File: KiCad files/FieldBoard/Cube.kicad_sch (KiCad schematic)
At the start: 9 parts

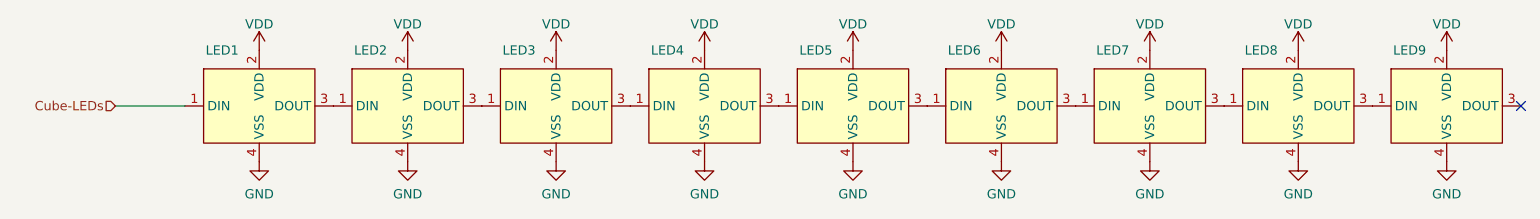
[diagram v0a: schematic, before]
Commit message: update
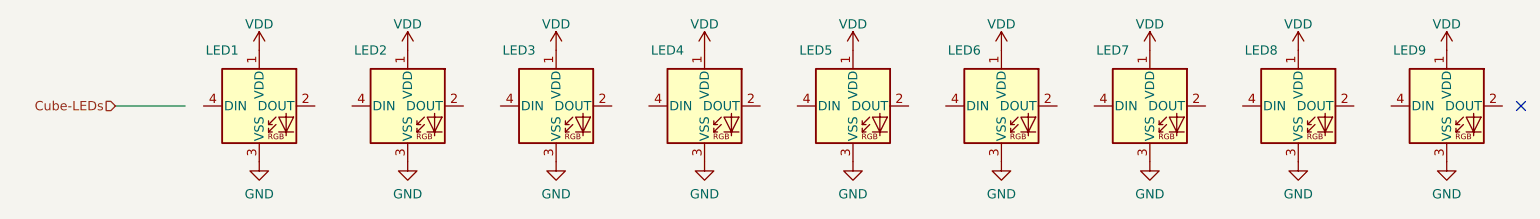
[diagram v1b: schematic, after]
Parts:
- LED1: value WS2812-4020_single -> (none); footprint FieldBoard_footprint:WS2812-4020-single-6mm_bezMaske -> LED_SMD:LED_WS2812B_PLCC4_5.0x5.0mm_P3.2mm; symbol FieldBoard_symbol:WS2812-4020_single -> LED:WS2812B
- LED2, LED3, LED4, LED5, LED6, LED7, LED8, LED9: footprint FieldBoard_footprint:WS2812-4020-single-6mm_bezMaske -> LED_SMD:LED_WS2812B_PLCC4_5.0x5.0mm_P3.2mm; symbol FieldBoard_symbol:WS2812-4020_single -> LED:WS2812B
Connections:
- net Cube-LEDs: no longer LED1.1 (DIN)
- net GND: now also LED1.3 (VSS), LED2.3 (VSS), LED3.3 (VSS), LED4.3 (VSS), LED5.3 (VSS), LED6.3 (VSS), LED7.3 (VSS), LED8.3 (VSS), LED9.3 (VSS); no longer LED1.4 (VSS), LED2.4 (VSS), LED3.4 (VSS), LED4.4 (VSS), LED5.4 (VSS), LED6.4 (VSS), LED7.4 (VSS), LED8.4 (VSS), LED9.4 (VSS)
- net VDD: now also LED1.1 (VDD), LED2.1 (VDD), LED3.1 (VDD), LED4.1 (VDD), LED5.1 (VDD), LED6.1 (VDD), LED7.1 (VDD), LED8.1 (VDD), LED9.1 (VDD); no longer LED1.2 (VDD), LED2.2 (VDD), LED3.2 (VDD), LED4.2 (VDD), LED5.2 (VDD), LED6.2 (VDD), LED7.2 (VDD), LED8.2 (VDD), LED9.2 (VDD)
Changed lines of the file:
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@@
     (pin "1")
   )
-  (symbol (lib_name "WS2812-4020_single_7") (lib_id "FieldBoard_symbol:WS2812-4020_single") (at 117.475 88.9 0) (unit 1)
+  (symbol (lib_id "LED:WS2812B") (at 117.475 88.9 0) (unit 1)
     (in_bom yes) (on_board yes)
     (property "Reference" "LED3" (id 0) (at 112.395 81.28 0))
@@
       (effects (font (size 1.27 1.27)) hide)
     )
-    (property "Footprint" "FieldBoard_footprint:WS2812-4020-single-6mm_bezMaske" (id 2) (at 117.475 88.9 0)
-      (effects (font (size 1.27 1.27)) hide)
-    )
-    (property "Datasheet" "" (id 3) (at 117.475 88.9 0)
-      (effects (font (size 1.27 1.27)) hide)
-    )
-    (pin "1")
-    (pin "2")
-    (pin "3")
-    (pin "4")
-  )
-  (symbol (lib_name "WS2812-4020_single_6") (lib_id "FieldBoard_symbol:WS2812-4020_single") (at 178.435 88.9 0) (unit 1)
+    (property "Footprint" "LED_SMD:LED_WS2812B_PLCC4_5.0x5.0mm_P3.2mm" (id 2) (at 118.745 96.52 0)
+      (effects (font (size 1.27 1.27)) (justify left top) hide)
+    )
+    (property "Datasheet" "https://cdn-shop.adafruit.com/datasheets/WS2812B.pdf" (id 3) (at 120.015 98.425 0)
+      (effects (font (size 1.27 1.27)) (justify left top) hide)
+    )
+    (pin "1")
+    (pin "2")
+    (pin "3")
+    (pin "4")
+  )
+  (symbol (lib_id "LED:WS2812B") (at 178.435 88.9 0) (unit 1)
     (in_bom yes) (on_board yes)
     (property "Reference" "LED6" (id 0) (at 173.355 81.28 0))
@@
       (effects (font (size 1.27 1.27)) hide)
     )
-    (property "Footprint" "FieldBoard_footprint:WS2812-4020-single-6mm_bezMaske" (id 2) (at 178.435 88.9 0)
-      (effects (font (size 1.27 1.27)) hide)
-    )
-    (property "Datasheet" "" (id 3) (at 178.435 88.9 0)
-      (effects (font (size 1.27 1.27)) hide)
-    )
-    (pin "1")
-    (pin "2")
-    (pin "3")
-    (pin "4")
-  )
-  (symbol (lib_name "WS2812-4020_single_2") (lib_id "FieldBoard_symbol:WS2812-4020_single") (at 97.155 88.9 0) (unit 1)
+    (property "Footprint" "LED_SMD:LED_WS2812B_PLCC4_5.0x5.0mm_P3.2mm" (id 2) (at 179.705 96.52 0)
+      (effects (font (size 1.27 1.27)) (justify left top) hide)
+    )
+    (property "Datasheet" "https://cdn-shop.adafruit.com/datasheets/WS2812B.pdf" (id 3) (at 180.975 98.425 0)
+      (effects (font (size 1.27 1.27)) (justify left top) hide)
+    )
+    (pin "1")
+    (pin "2")
+    (pin "3")
+    (pin "4")
+  )
+  (symbol (lib_id "LED:WS2812B") (at 97.155 88.9 0) (unit 1)
     (in_bom yes) (on_board yes)
     (property "Reference" "LED2" (id 0) (at 92.075 81.28 0))
@@
       (effects (font (size 1.27 1.27)) hide)
     )
-    (property "Footprint" "FieldBoard_footprint:WS2812-4020-single-6mm_bezMaske" (id 2) (at 97.155 88.9 0)
-      (effects (font (size 1.27 1.27)) hide)
-    )
-    (property "Datasheet" "" (id 3) (at 97.155 88.9 0)
-      (effects (font (size 1.27 1.27)) hide)
+    (property "Footprint" "LED_SMD:LED_WS2812B_PLCC4_5.0x5.0mm_P3.2mm" (id 2) (at 98.425 96.52 0)
+      (effects (font (size 1.27 1.27)) (justify left top) hide)
+    )
+    (property "Datasheet" "https://cdn-shop.adafruit.com/datasheets/WS2812B.pdf" (id 3) (at 99.695 98.425 0)
+      (effects (font (size 1.27 1.27)) (justify left top) hide)
     )
     (pin "1")
@@
     (pin "1")
   )
-  (symbol (lib_name "WS2812-4020_single_3") (lib_id "FieldBoard_symbol:WS2812-4020_single") (at 239.395 88.9 0) (unit 1)
+  (symbol (lib_id "LED:WS2812B") (at 239.395 88.9 0) (unit 1)
     (in_bom yes) (on_board yes)
     (property "Reference" "LED9" (id 0) (at 234.315 81.28 0))
@@
       (effects (font (size 1.27 1.27)) hide)
     )
-    (property "Footprint" "FieldBoard_footprint:WS2812-4020-single-6mm_bezMaske" (id 2) (at 239.395 88.9 0)
-      (effects (font (size 1.27 1.27)) hide)
-    )
-    (property "Datasheet" "" (id 3) (at 239.395 88.9 0)
-      (effects (font (size 1.27 1.27)) hide)
+    (property "Footprint" "LED_SMD:LED_WS2812B_PLCC4_5.0x5.0mm_P3.2mm" (id 2) (at 240.665 96.52 0)
+      (effects (font (size 1.27 1.27)) (justify left top) hide)
+    )
+    (property "Datasheet" "https://cdn-shop.adafruit.com/datasheets/WS2812B.pdf" (id 3) (at 241.935 98.425 0)
+      (effects (font (size 1.27 1.27)) (justify left top) hide)
     )
     (pin "1")
@@
     (pin "1")
   )
-  (symbol (lib_id "FieldBoard_symbol:WS2812-4020_single") (at 158.115 88.9 0) (unit 1)
+  (symbol (lib_id "LED:WS2812B") (at 158.115 88.9 0) (unit 1)
     (in_bom yes) (on_board yes)
     (property "Reference" "LED5" (id 0) (at 153.035 81.28 0))
@@
       (effects (font (size 1.27 1.27)) hide)
     )
-    (property "Footprint" "FieldBoard_footprint:WS2812-4020-single-6mm_bezMaske" (id 2) (at 158.115 88.9 0)
-      (effects (font (size 1.27 1.27)) hide)
-    )
-    (property "Datasheet" "" (id 3) (at 158.115 88.9 0)
-      (effects (font (size 1.27 1.27)) hide)
+    (property "Footprint" "LED_SMD:LED_WS2812B_PLCC4_5.0x5.0mm_P3.2mm" (id 2) (at 159.385 96.52 0)
+      (effects (font (size 1.27 1.27)) (justify left top) hide)
+    )
+    (property "Datasheet" "https://cdn-shop.adafruit.com/datasheets/WS2812B.pdf" (id 3) (at 160.655 98.425 0)
+      (effects (font (size 1.27 1.27)) (justify left top) hide)
     )
     (pin "1")
@@
     (pin "1")
   )
-  (symbol (lib_name "WS2812-4020_single_4") (lib_id "FieldBoard_symbol:WS2812-4020_single") (at 219.075 88.9 0) (unit 1)
+  (symbol (lib_id "LED:WS2812B") (at 219.075 88.9 0) (unit 1)
     (in_bom yes) (on_board yes)
     (property "Reference" "LED8" (id 0) (at 213.995 81.28 0))
@@
       (effects (font (size 1.27 1.27)) hide)
     )
-    (property "Footprint" "FieldBoard_footprint:WS2812-4020-single-6mm_bezMaske" (id 2) (at 219.075 88.9 0)
-      (effects (font (size 1.27 1.27)) hide)
-    )
-    (property "Datasheet" "" (id 3) (at 219.075 88.9 0)
-      (effects (font (size 1.27 1.27)) hide)
-    )
-    (pin "1")
-    (pin "2")
-    (pin "3")
-    (pin "4")
-  )
-  (symbol (lib_name "WS2812-4020_single_1") (lib_id "FieldBoard_symbol:WS2812-4020_single") (at 76.835 88.9 0) (unit 1)
+    (property "Footprint" "LED_SMD:LED_WS2812B_PLCC4_5.0x5.0mm_P3.2mm" (id 2) (at 220.345 96.52 0)
+      (effects (font (size 1.27 1.27)) (justify left top) hide)
+    )
+    (property "Datasheet" "https://cdn-shop.adafruit.com/datasheets/WS2812B.pdf" (id 3) (at 221.615 98.425 0)
+      (effects (font (size 1.27 1.27)) (justify left top) hide)
+    )
+    (pin "1")
+    (pin "2")
+    (pin "3")
+    (pin "4")
+  )
+  (symbol (lib_id "LED:WS2812B") (at 76.835 88.9 0) (unit 1)
     (in_bom yes) (on_board yes)
     (property "Reference" "LED1" (id 0) (at 71.755 81.28 0))
-    (property "Value" "WS2812-4020_single" (id 1) (at 86.995 96.52 0)
-      (effects (font (size 1.27 1.27)) hide)
-    )
-    (property "Footprint" "FieldBoard_footprint:WS2812-4020-single-6mm_bezMaske" (id 2) (at 76.835 88.9 0)
-      (effects (font (size 1.27 1.27)) hide)
-    )
-    (property "Datasheet" "" (id 3) (at 76.835 88.9 0)
-      (effects (font (size 1.27 1.27)) hide)
+    (property "Value" "" (id 1) (at 86.995 96.52 0)
+      (effects (font (size 1.27 1.27)) hide)
+    )
+    (property "Footprint" "LED_SMD:LED_WS2812B_PLCC4_5.0x5.0mm_P3.2mm" (id 2) (at 78.105 96.52 0)
+      (effects (font (size 1.27 1.27)) (justify left top) hide)
+    )
+    (property "Datasheet" "https://cdn-shop.adafruit.com/datasheets/WS2812B.pdf" (id 3) (at 79.375 98.425 0)
+      (effects (font (size 1.27 1.27)) (justify left top) hide)
     )
     (pin "1")
@@
     (pin "1")
   )
-  (symbol (lib_name "WS2812-4020_single_5") (lib_id "FieldBoard_symbol:WS2812-4020_single") (at 198.755 88.9 0) (unit 1)
+  (symbol (lib_id "LED:WS2812B") (at 198.755 88.9 0) (unit 1)
     (in_bom yes) (on_board yes)
     (property "Reference" "LED7" (id 0) (at 193.675 81.28 0))
@@
       (effects (font (size 1.27 1.27)) hide)
     )
-    (property "Footprint" "FieldBoard_footprint:WS2812-4020-single-6mm_bezMaske" (id 2) (at 198.755 88.9 0)
-      (effects (font (size 1.27 1.27)) hide)
-    )
-    (property "Datasheet" "" (id 3) (at 198.755 88.9 0)
-      (effects (font (size 1.27 1.27)) hide)
+    (property "Footprint" "LED_SMD:LED_WS2812B_PLCC4_5.0x5.0mm_P3.2mm" (id 2) (at 200.025 96.52 0)
+      (effects (font (size 1.27 1.27)) (justify left top) hide)
+    )
+    (property "Datasheet" "https://cdn-shop.adafruit.com/datasheets/WS2812B.pdf" (id 3) (at 201.295 98.425 0)
+      (effects (font (size 1.27 1.27)) (justify left top) hide)
     )
     (pin "1")
@@
     (pin "1")
   )
-  (symbol (lib_name "WS2812-4020_single_8") (lib_id "FieldBoard_symbol:WS2812-4020_single") (at 137.795 88.9 0) (unit 1)
+  (symbol (lib_id "LED:WS2812B") (at 137.795 88.9 0) (unit 1)
     (in_bom yes) (on_board yes)
     (property "Reference" "LED4" (id 0) (at 132.715 81.28 0))
@@
       (effects (font (size 1.27 1.27)) hide)
     )
-    (property "Footprint" "FieldBoard_footprint:WS2812-4020-single-6mm_bezMaske" (id 2) (at 137.795 88.9 0)
-      (effects (font (size 1.27 1.27)) hide)
-    )
-    (property "Datasheet" "" (id 3) (at 137.795 88.9 0)
-      (effects (font (size 1.27 1.27)) hide)
-    )
-    (pin "1")
+    (property "Footprint" "LED_SMD:LED_WS2812B_PLCC4_5.0x5.0mm_P3.2mm" (id 2) (at 139.065 96.52 0)
+      (effects (font (size 1.27 1.27)) (justify left top) hide)
+    )
+    (property "Datasheet" "https://cdn-shop.adafruit.com/datasheets/WS2812B.pdf" (id 3) (at 140.335 98.425 0)
+      (effects (font (size 1.27 1.27)) (justify left top) hide)
+    )
+    (pin "1")
